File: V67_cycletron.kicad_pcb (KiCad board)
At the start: 4 copper layers, 112.9 x 44.8 mm, 54 parts, among them J1 USB_C_Receptacle_USB2.0_16P, J2 Conn_01x04_Socket, J3 Conn_01x04_Socket, U2 LM1117DT-3.3, U3 L7805, U4 ESP32-S3-WROOM-1

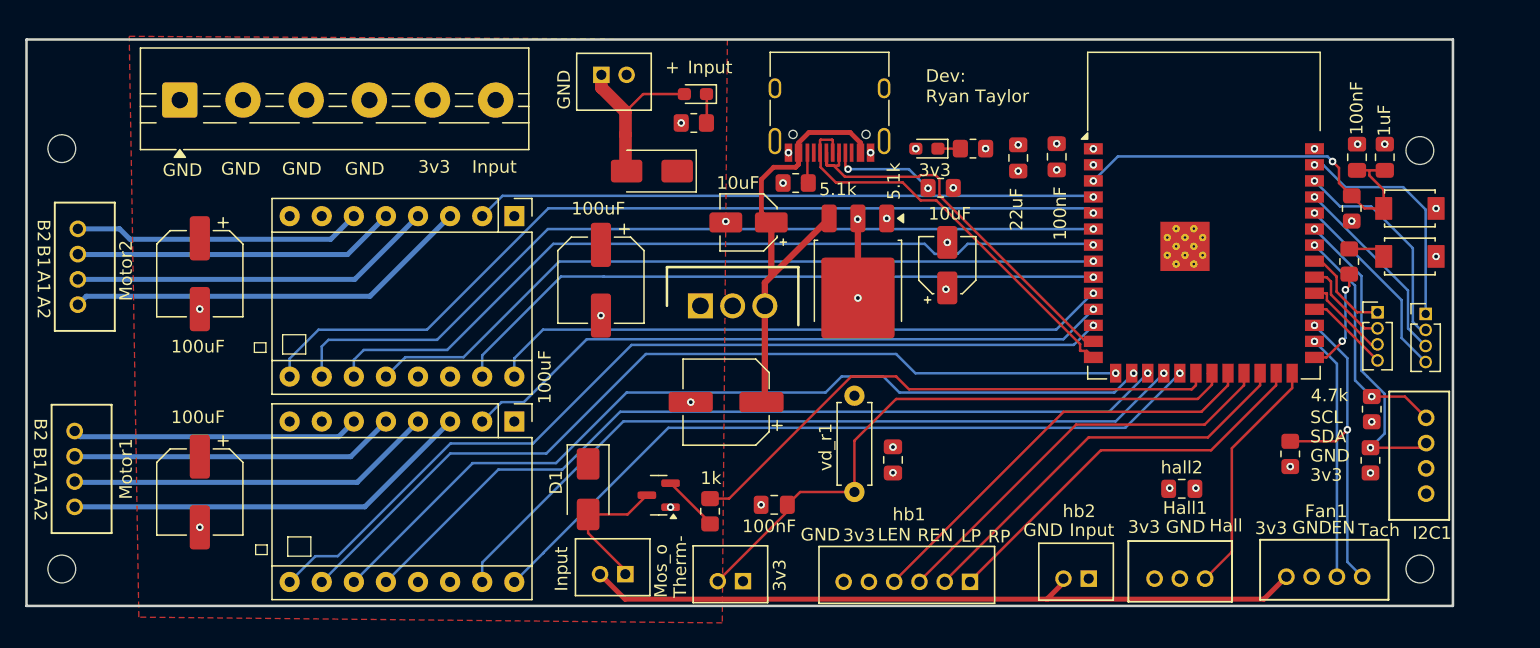
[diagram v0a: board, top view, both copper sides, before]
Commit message: big changes to make it work
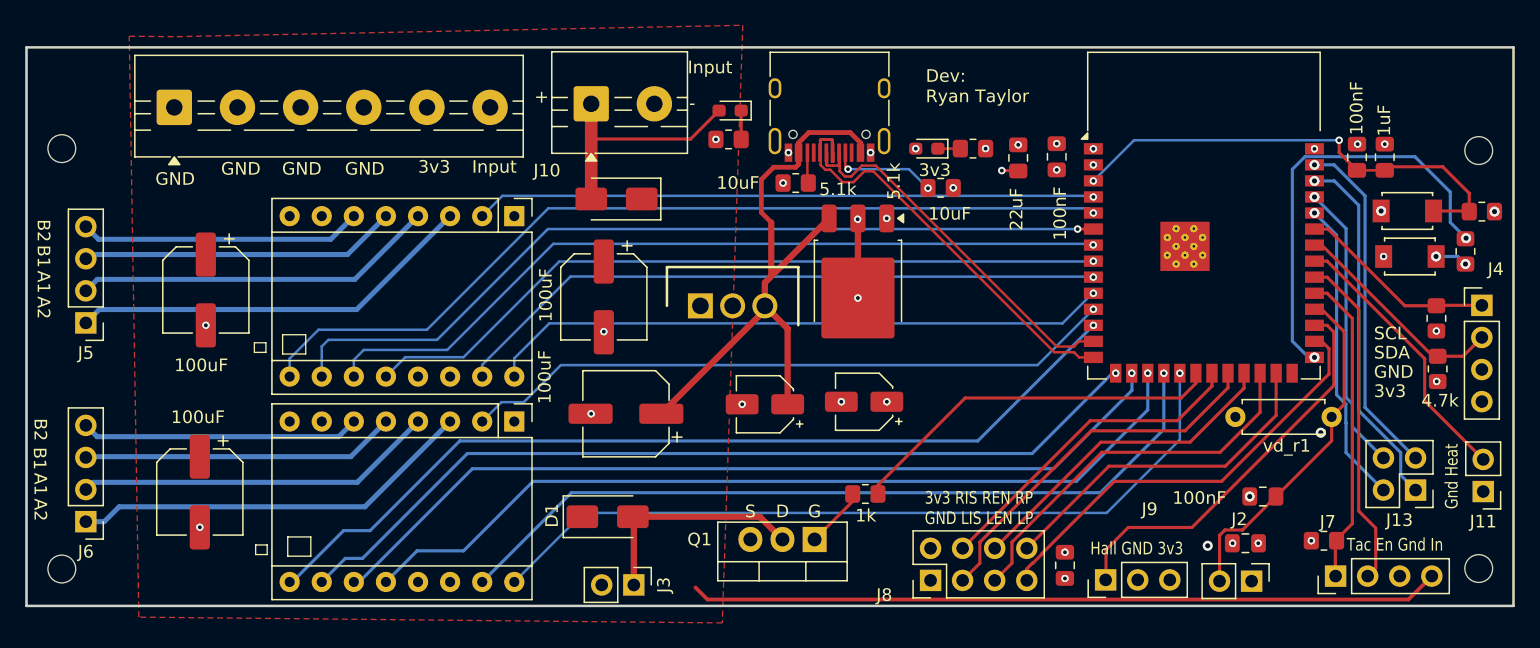
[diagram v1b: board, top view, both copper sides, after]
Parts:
- removed Fan1: PC_Fan, connector_4_vert:CONN4_B4B-PH_JST
- removed Hall1: Hall_Sens, connector_3_vert:CONN_B3B-PH-K-SLFSN_JST
- removed I2C1: MCP9600, connector_4_vert:CONN4_B4B-PH_JST
- removed Input1, Mos1, Therm1, hb2: B2B-PH-K-S, connector_2_vert:JST_B2B-PH-K-S
- removed Motor1: Motor1, connector_4_vert:CONN4_B4B-PH_JST
- removed Motor2: Motor2, connector_4_vert:CONN4_B4B-PH_JST
- removed hb1: B6B-PH-K-S, connector_6_vert:JST_B6B-PH-K-S
- removed mosfet4: HD2305, Package_TO_SOT_SMD:SOT-23
- added J10: Screw_Terminal_01x02, TerminalBlock:TerminalBlock_MaiXu_MX126-5.0-02P_1x02_P5.00mm, F.Cu at (80.0, 76.7)
- added J11: PINHD_1x2_Male, Connector_PinHeader_2.54mm:PinHeader_1x02_P2.54mm_Vertical, F.Cu at (150.6, 107.4)
- added J13: PINHD_2x2_Male, Connector_PinHeader_2.54mm:PinHeader_2x02_P2.54mm_Vertical, F.Cu at (145.2, 107.3)
- added J4: PINHD_1x4_Male, Connector_PinHeader_2.54mm:PinHeader_1x04_P2.54mm_Vertical, F.Cu at (150.5, 92.7)
- added J5: PINHD_1x4_Male, Connector_PinHeader_2.54mm:PinHeader_1x04_P2.54mm_Vertical, F.Cu at (40.0, 94.1)
- added J6: PINHD_1x4_Male, Connector_PinHeader_2.54mm:PinHeader_1x04_P2.54mm_Vertical, F.Cu at (40.0, 109.8)
- added J7: PINHD_1x4_Male, Connector_PinHeader_2.54mm:PinHeader_1x04_P2.54mm_Vertical, F.Cu at (138.9, 114.1)
- added J8: PINHD_2x4_Male, Connector_PinHeader_2.54mm:PinHeader_2x04_P2.54mm_Vertical, F.Cu at (106.9, 114.4)
- added J9: PINHD_1x3_Male, Connector_PinHeader_2.54mm:PinHeader_1x03_P2.54mm_Vertical, F.Cu at (120.7, 114.4)
- added Q1: IRF1324, PCM_Package_TO_SOT_THT_AKL:TO-220-3_Vertical_GDS, F.Cu at (97.7, 111.2)
- D4, D5: value LED -> LED_RED
- J2, J3: value Conn_01x04_Socket -> PINHD_1x2_Male; footprint Connector_PinHeader_1.27mm:PinHeader_1x04_P1.27mm_Vertical -> Connector_PinHeader_2.54mm:PinHeader_1x02_P2.54mm_Vertical
- moved J3 62.7 mm to (83.4, 114.8), turned to -90 degrees
- moved vd_c2 38.7 mm to (133.2, 107.8)
- moved vd_r1 38.2 mm to (138.6, 101.5), turned to 180 degrees
- moved vd_c1 28.7 mm to (131.8, 111.5), turned to 180 degrees
- moved J2 25.2 mm to (132.3, 114.5), turned to -90 degrees
- moved 5Vout1 14.5 mm to (93.8, 100.5)
- moved 3v3out1 12.7 mm to (101.6, 100.3), turned to 180 degrees
- moved tr3 12.4 mm to (101.7, 107.6), turned to 0 degrees
- moved hall2 11.1 mm to (117.5, 113.2), turned to 90 degrees
- moved R_En1 10.3 mm to (150.5, 85.2), turned to 180 degrees
- moved R_boot1 9.23 mm to (149.2, 88.4), turned to 90 degrees
- moved R5 8.98 mm to (147.0, 97.7)
- moved R4 8.82 mm to (146.9, 93.7)
- moved 3v3in1 7.98 mm to (82.8, 101.2)
- moved R7 7.37 mm to (138.0, 111.3), turned to 0 degrees
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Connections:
- J2 pad 1: IO1 -> 3V3
- J2 pad 2: IO2 -> Therm-
- J3 pad 1: IO40 -> mosfet1_o
- J3 pad 2: IO39 -> +24V
- U4 pad 21: Therm- -> R_IS
- U4 pad 22: L_EN -> L_IS
- U4 pad 24: LPWM -> L_EN
- U4 pad 26: Hall_i -> unconnected-(U4-IO45-Pad26)
- U4 pad 28: FAN_En_o -> LPWM
- U4 pad 29: FAN_Tach_i -> Hall_i
- U4 pad 30: IO37 -> Therm-
- U4 pad 31: IO38 -> FAN_Tach_i
- U4 pad 32: IO39 -> FAN_En_o
- U4 pad 33: IO40 -> Heat_o
- U4 pad 34: SCL -> SDA
- U4 pad 35: SDA -> SCL
- tr3 pad 1: mosfet1_i -> Net-(Q1-G)
- tr3 pad 2: Net-(mosfet4-G) -> mosfet1_i
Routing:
- net L_IS: track 0.00 -> 29.4 mm
- net R_IS: track 0.00 -> 26.2 mm
- net BOOT: track 8.71 -> 34.3 mm
- net Heat_o: track 0.00 -> 21.8 mm
- net Therm-: track 49.3 -> 27.7 mm
- net mosfet1_i: track 44.0 -> 30.0 mm
- net +5V: track 36.3 -> 49.1 mm
- net Hall_i: track 19.1 -> 31.8 mm
- net IO2: track 17.1 -> 28.7 mm
- net IO1: track 18.5 -> 27.4 mm
- net RX: track 15.4 -> 24.2 mm
- net TX: track 15.4 -> 22.9 mm
- net IO40: track 7.37 -> 0.00 mm
- net IO39: track 7.27 -> 0.00 mm
- net FAN_En_o: track 19.4 -> 26.5 mm, vias 1 -> 0
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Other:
- board size 112.9 x 44.8 mm -> 117.7 x 44.2 mm
- board text added: "-"
- board text added: "3v3 RIS REN RP GND LIS LEN LP"
- board text added: "Gnd Heat"
- board text added: "Hall GND 3v3"
- board text added: "Tac En Gnd In"
- board text removed: "EN"
- board text removed: "Hall"
- board text removed: "LEN"
- board text removed: "LP"
- board text removed: "Mos_o"
- board text removed: "REN"
- board text removed: "RP"
- board text removed: "Tach"
- board text removed: "Therm-"
